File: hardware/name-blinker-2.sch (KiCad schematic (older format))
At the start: 47 parts, among them M1 MOUNTING-HOLE, M10 MOUNTING-HOLE, M11 MOUNTING-HOLE, M12 MOUNTING-HOLE, M13 MOUNTING-HOLE, M2 MOUNTING-HOLE, M3 MOUNTING-HOLE, M4 MOUNTING-HOLE, M5 MOUNTING-HOLE, M6 MOUNTING-HOLE, M7 MOUNTING-HOLE, M8 MOUNTING-HOLE, M9 MOUNTING-HOLE, P1 CONN_01X09, P2 USB_OTG, SW2 SMD-TOGGLE-SWITCH-2CH_2X3P-7X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, U1 MCP73831, U2 BMD-300, U3 TPS63051

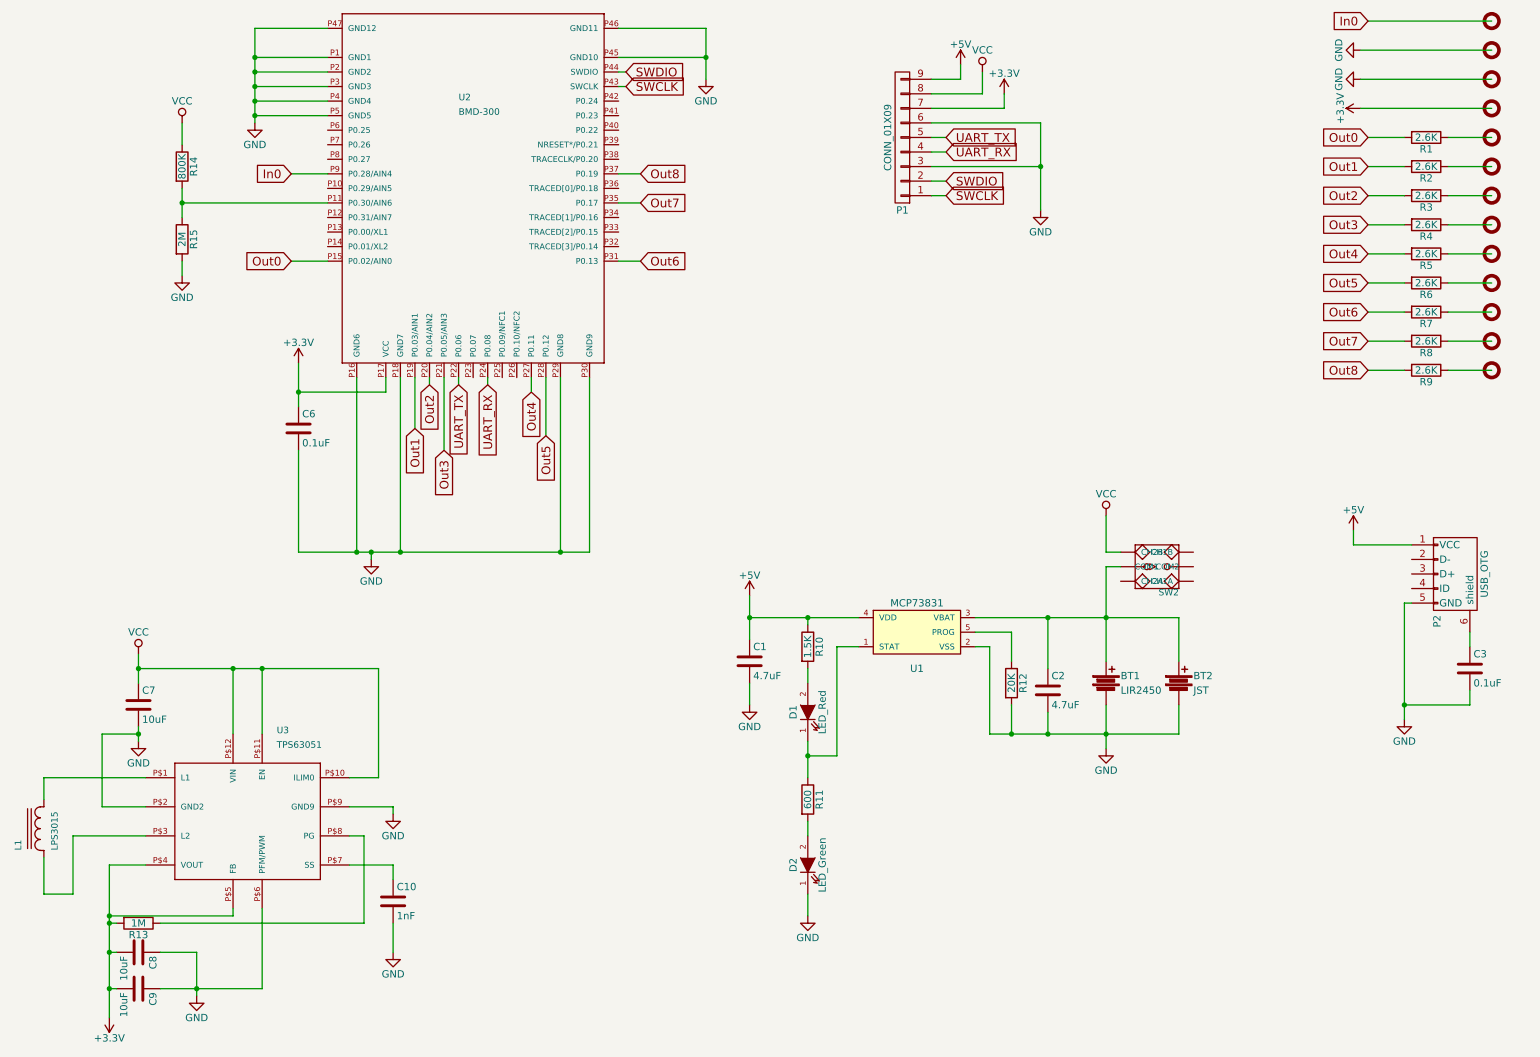
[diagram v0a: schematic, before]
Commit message: connected everything
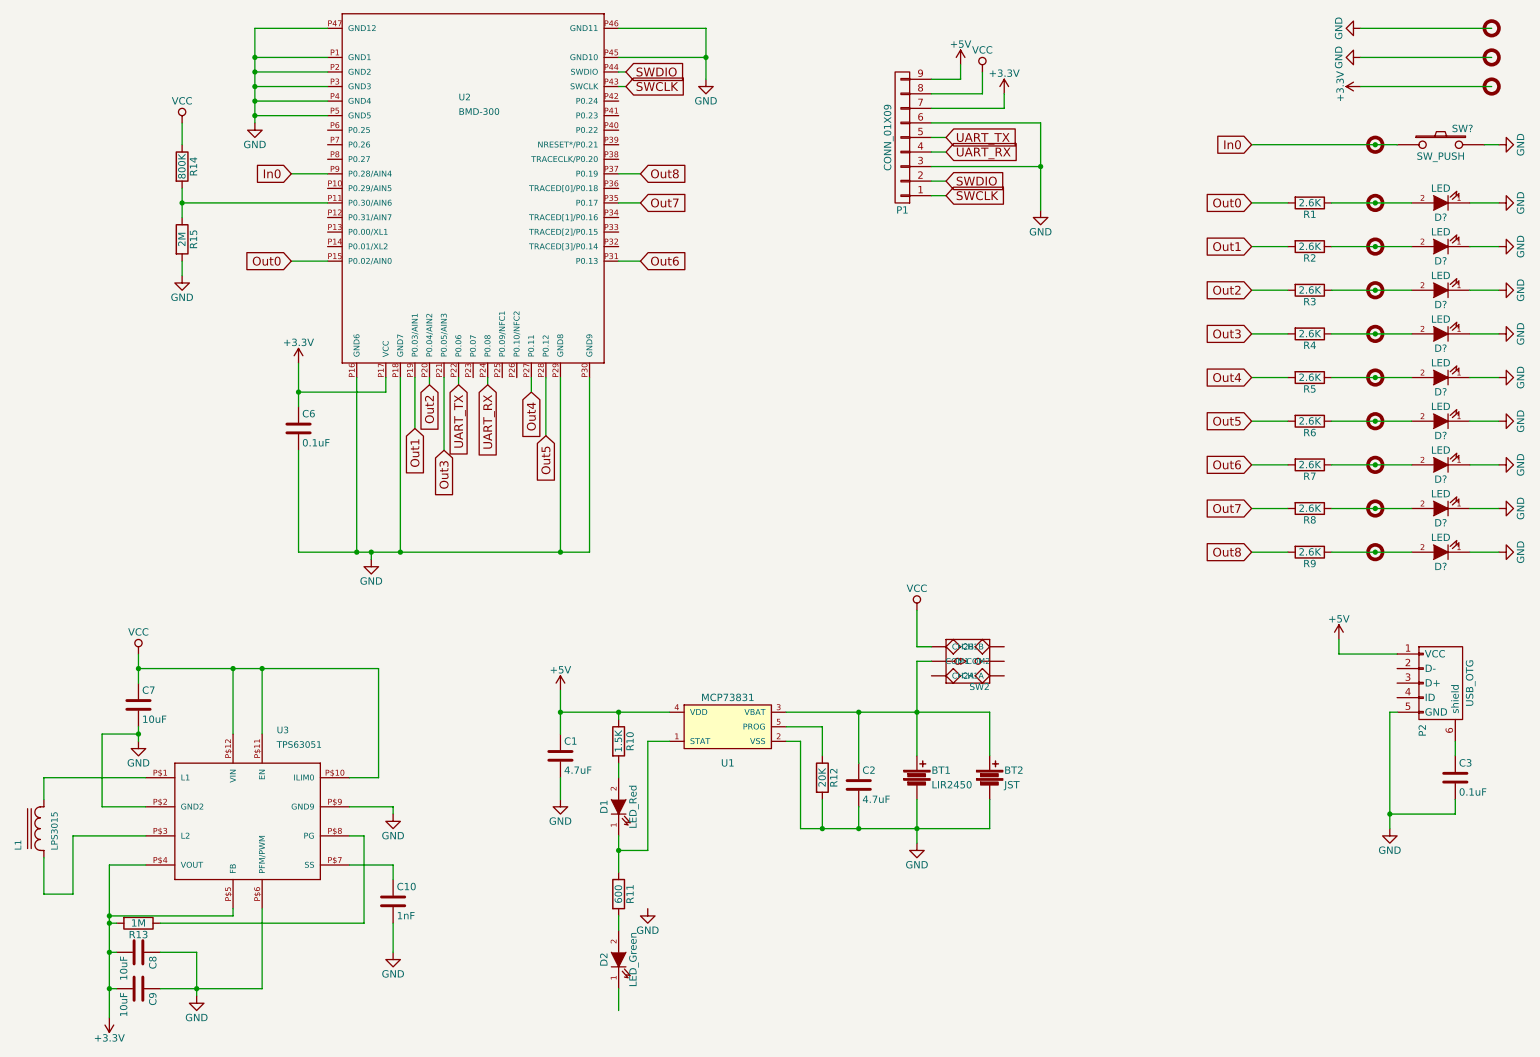
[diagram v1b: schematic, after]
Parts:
- added D? (x9): LED, symbol LED
- added SW?: SW_PUSH, symbol SW_PUSH
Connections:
- net GND: now also D?.1 (K), D?.1 (K), D?.1 (K), D?.1 (K), D?.1 (K), D?.1 (K), D?.1 (K), D?.1 (K), D?.1 (K), SW?.2; no longer D2.1 (K)
- net In0: now also SW?.1
- net at M2.1, R1.1: now also D?.2 (A)
- net at M3.1, R2.1: now also D?.2 (A)
- net at M4.1, R3.1: now also D?.2 (A)
- net at M5.1, R4.1: now also D?.2 (A)
- net at M6.1, R5.1: now also D?.2 (A)
- net at M7.1, R6.1: now also D?.2 (A)
- net at M8.1, R7.1: now also D?.2 (A)
- net at M9.1, R8.1: now also D?.2 (A)
- net at M10.1, R9.1: now also D?.2 (A)
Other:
- moved on the sheet: BT1, BT2, C1, C2, C3, D1, D2, P2, R1, R10, R11, R12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
